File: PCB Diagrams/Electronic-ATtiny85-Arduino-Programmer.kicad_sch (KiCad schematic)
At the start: 6 parts, among them J1 POWER, J2 01x03, J3 01x01, U1 Arduino Nano v3.x, U2 ATtiny85

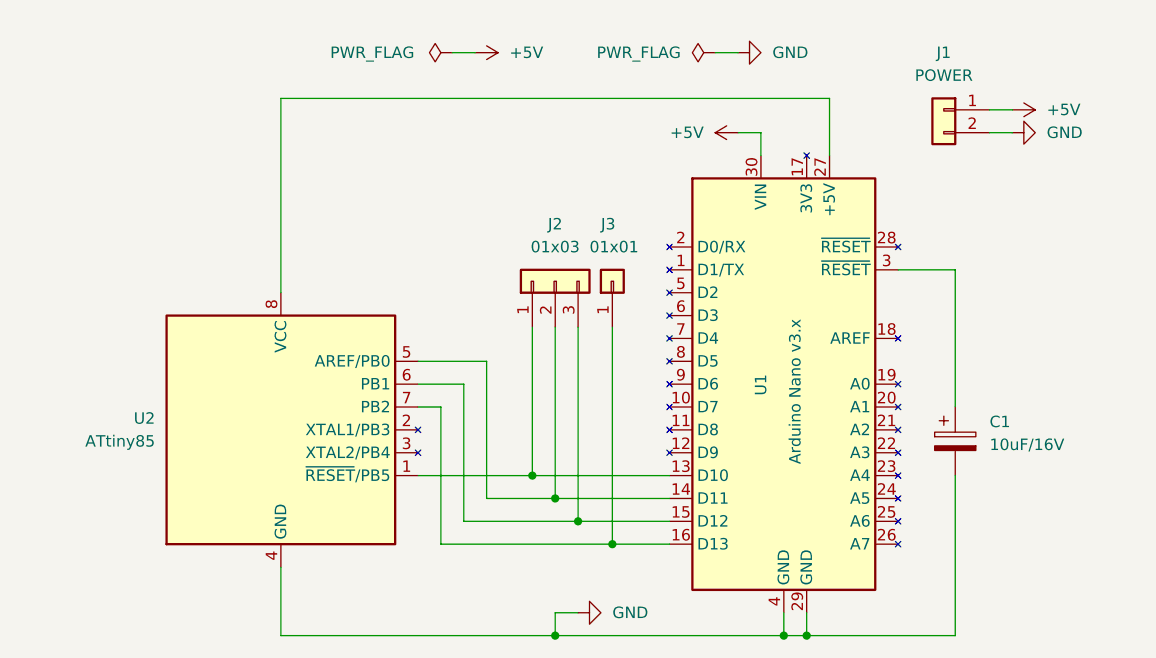
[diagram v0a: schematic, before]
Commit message: fixed PCB bug
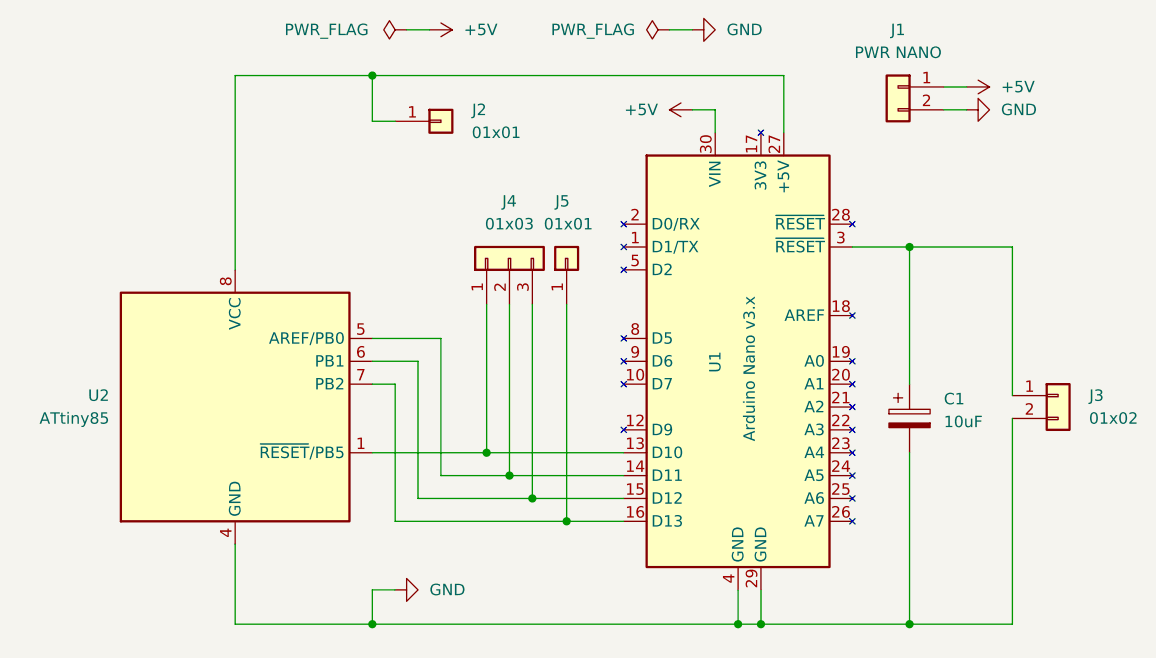
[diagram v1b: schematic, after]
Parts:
- added J2: 01x01, Connector_PinHeader_2.54mm:PinHeader_1x01_P2.54mm_Vertical, symbol Connector_Generic:Conn_01x01
- added J3: 01x02, Connector_PinHeader_2.54mm:PinHeader_1x02_P2.54mm_Vertical, symbol Connector_Generic:Conn_01x02
- C1: value 10uF/16V -> 10uF
- J1: value POWER -> PWR NANO
- J4: renamed from J2; footprint Connector_PinSocket_2.54mm:PinSocket_1x03_P2.54mm_Vertical -> Connector_PinHeader_2.54mm:PinHeader_1x03_P2.54mm_Vertical
- J5: renamed from J3; footprint Connector_PinSocket_2.54mm:PinSocket_1x01_P2.54mm_Vertical -> Connector_PinHeader_2.54mm:PinHeader_1x01_P2.54mm_Vertical
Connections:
- net GND: now also J3.2 (Pin_2)
- net at U1.27 (+5V), U2.8 (VCC): now also J2.1 (Pin_1)
- net at C1.1, U1.3 (~{RESET}): now also J3.1 (Pin_1)
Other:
- moved on the sheet: C1, J1, J4, J5
